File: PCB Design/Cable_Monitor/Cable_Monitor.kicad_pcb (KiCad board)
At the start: 2 copper layers, 63.5 x 118.1 mm, 43 parts, among them P1 type="R" model="Conn_01x32_Fe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, P2 type="R" model="Conn_01x32_Fe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, Q1 BSS316N, SW1 type="R" model="SW_Push" lib=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, U1 SiP32508, U2 LD1117S33TR, U3 MCP6002-xSN, U4 MCP6002-xSN, U5 DRV5053_SMD, U6 DRV5053_SMD, U8 type="R" model="DRV5053_THT" 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, Y1 OpenLog, Y2 Radar K-LC5-RFB-00C

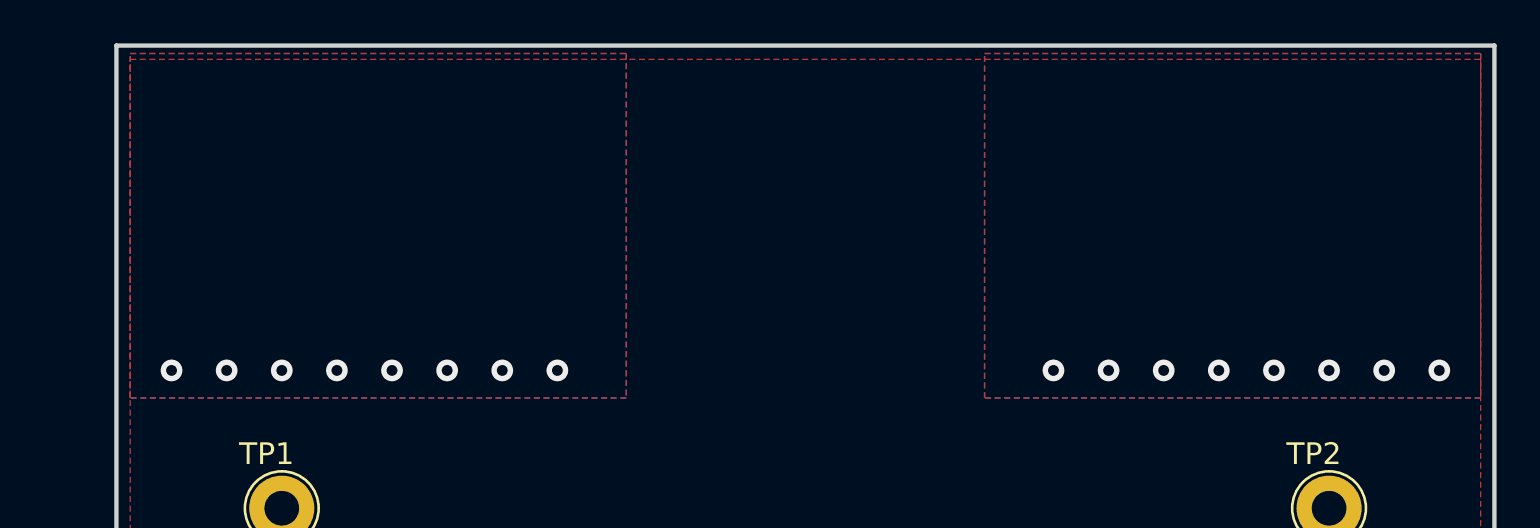
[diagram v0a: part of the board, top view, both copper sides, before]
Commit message: PCB Design Update
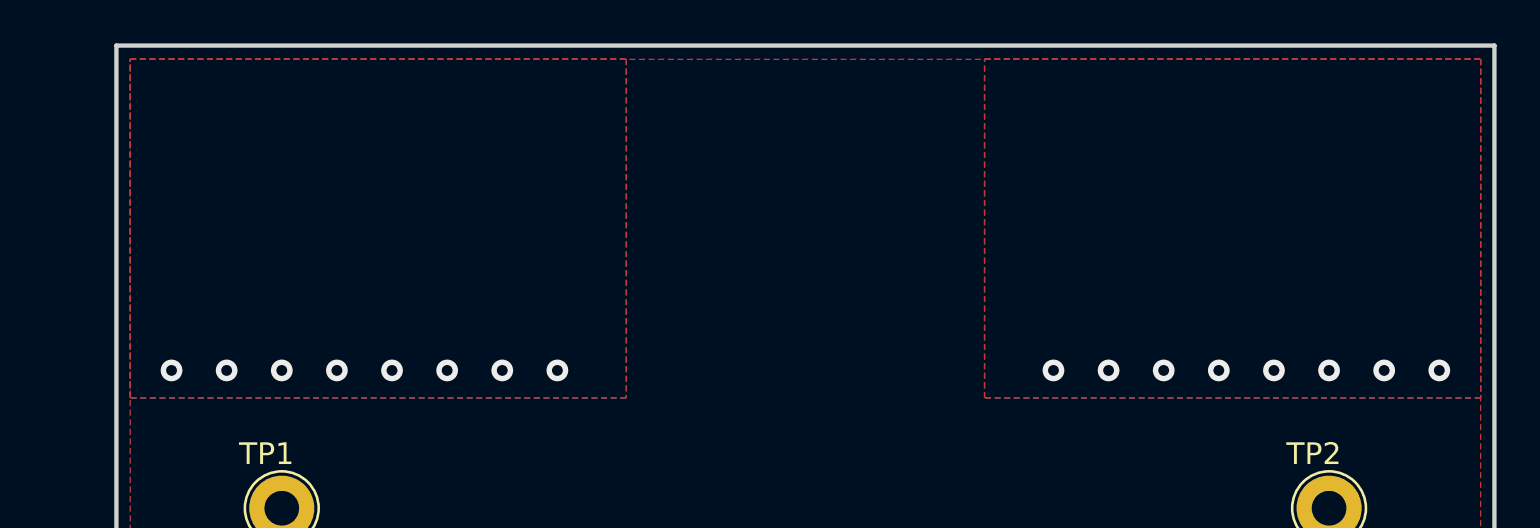
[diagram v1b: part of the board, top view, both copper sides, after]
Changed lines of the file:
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@@
         (xy 127.635 49.53)
         (xy 104.775 49.53)
-        (xy 104.775 33.655)
-        (xy 127.635 33.655)
+        (xy 104.775 33.909)
+        (xy 127.635 33.909)
       )
     )
@@
         (xy 167.005 49.53)
         (xy 144.145 49.53)
-        (xy 144.145 33.655)
-        (xy 167.005 33.655)
+        (xy 144.145 33.909)
+        (xy 167.005 33.909)
       )
     )
